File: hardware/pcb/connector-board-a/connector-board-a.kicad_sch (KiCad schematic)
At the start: 22 parts, among them J1 DE9_Pins, J2 8-215570-0, Q3 2N7002, U4 TPS63001

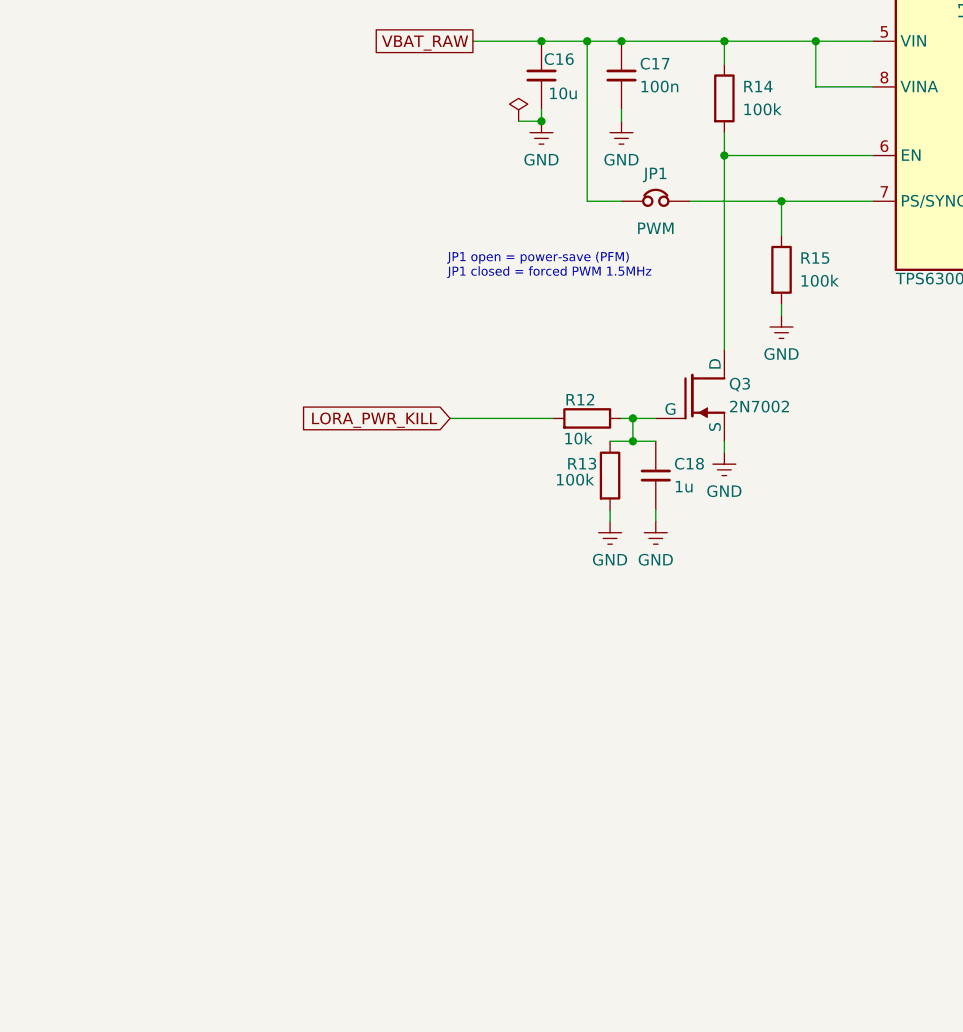
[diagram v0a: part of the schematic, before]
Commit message: Cleanup
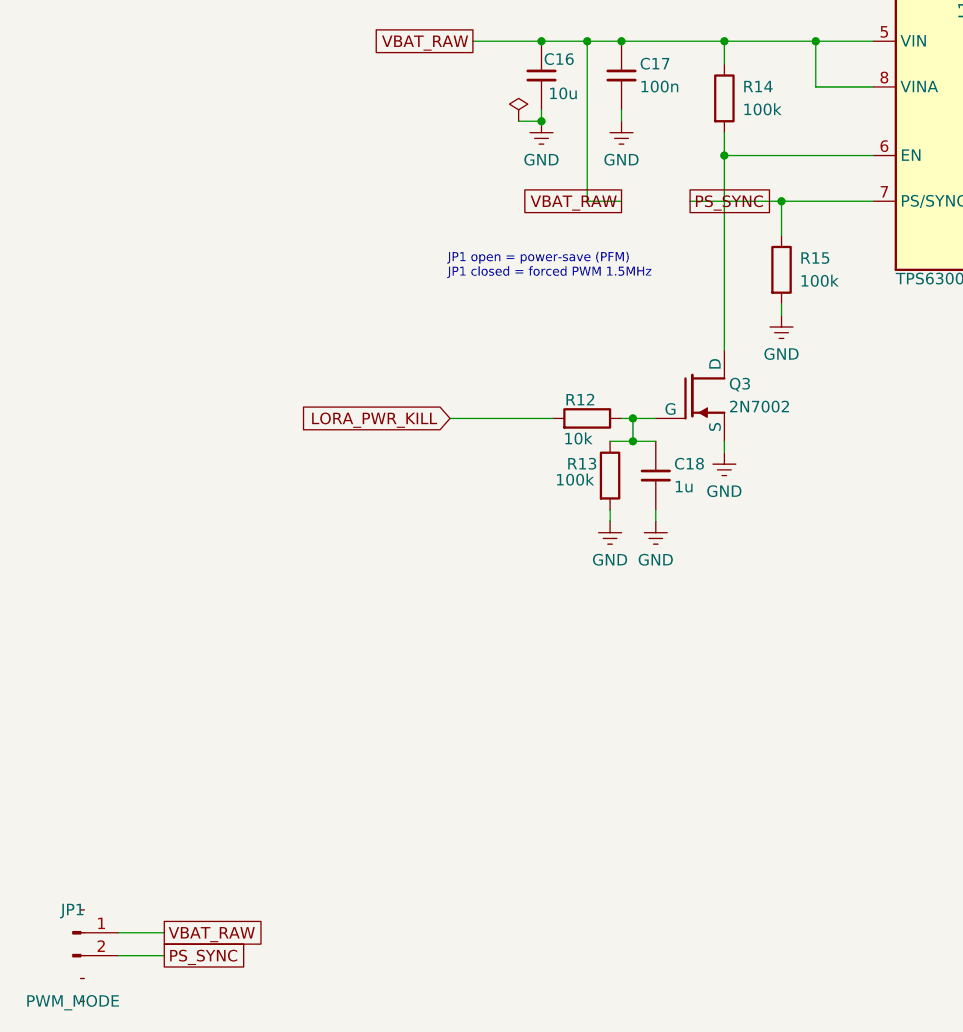
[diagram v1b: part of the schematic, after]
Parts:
- removed JP1: PWM, Jumper:SolderJumper-2_P1.3mm_Open_RoundedPad1.0x1.5mm, symbol lora3v3:JUMPER_H
- added JP1: PWM_MODE, Connector_PinHeader_2.54mm:PinHeader_1x02_P2.54mm_Vertical, symbol Connector:Conn_01x02_Pin
- J2: footprint TwinOak platform footprints:82155700 -> TwinOak:82155700; symbol 8-215570-0:8-215570-0 -> TwinOak:8-215570-0
- U4: symbol lora3v3:TPS63001 -> TwinOak:TPS63001
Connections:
- net VBAT_RAW: now also JP1.1 (Pin_1)
- net PS_SYNC: now reaches R15.1, U4.7 (PS/SYNC)
- net PS_SYNC: now also JP1.2 (Pin_2)
